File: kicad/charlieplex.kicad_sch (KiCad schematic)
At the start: 244 parts

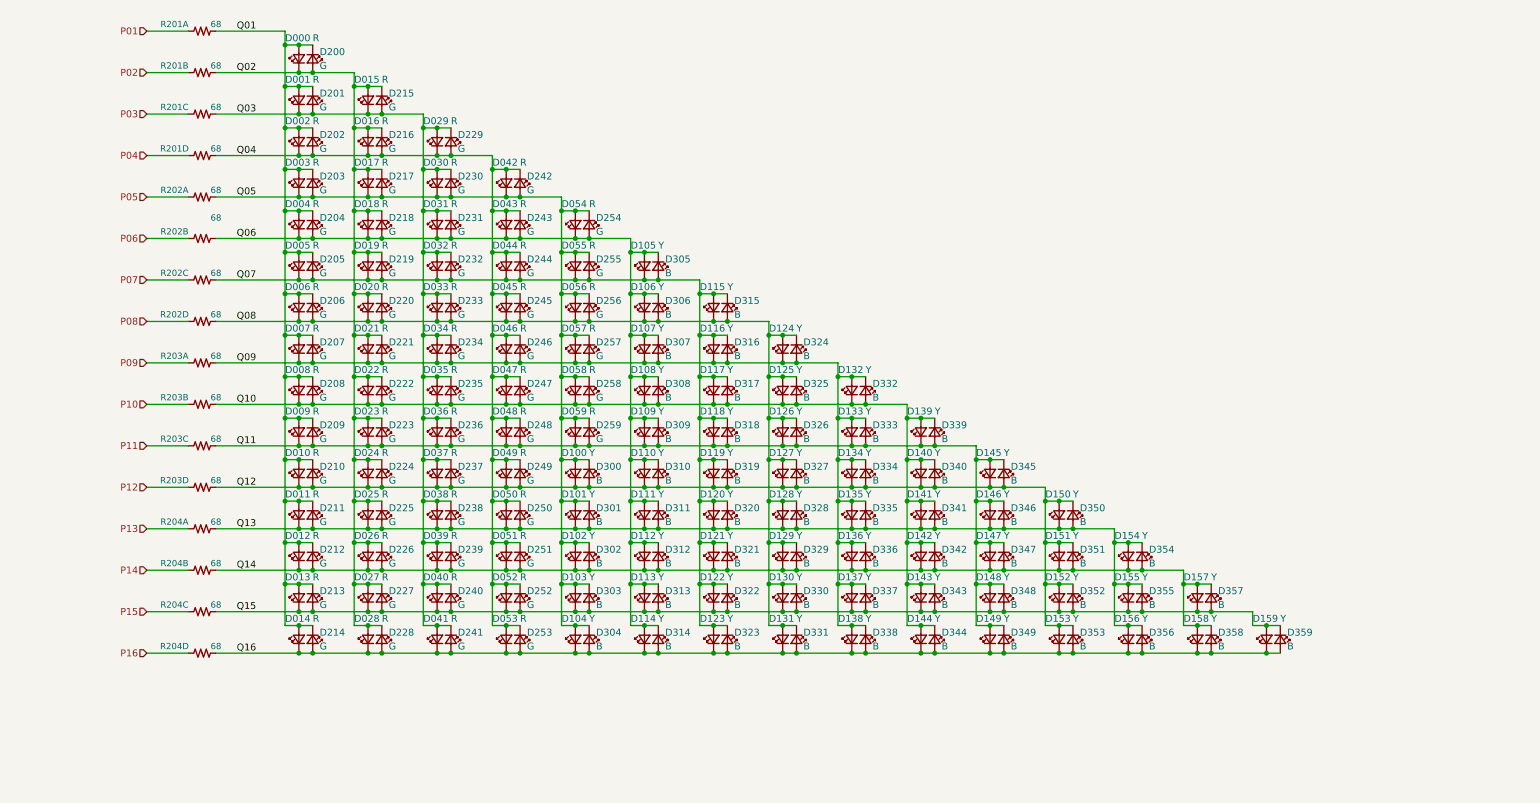
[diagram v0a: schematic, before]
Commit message: Lots of stuff
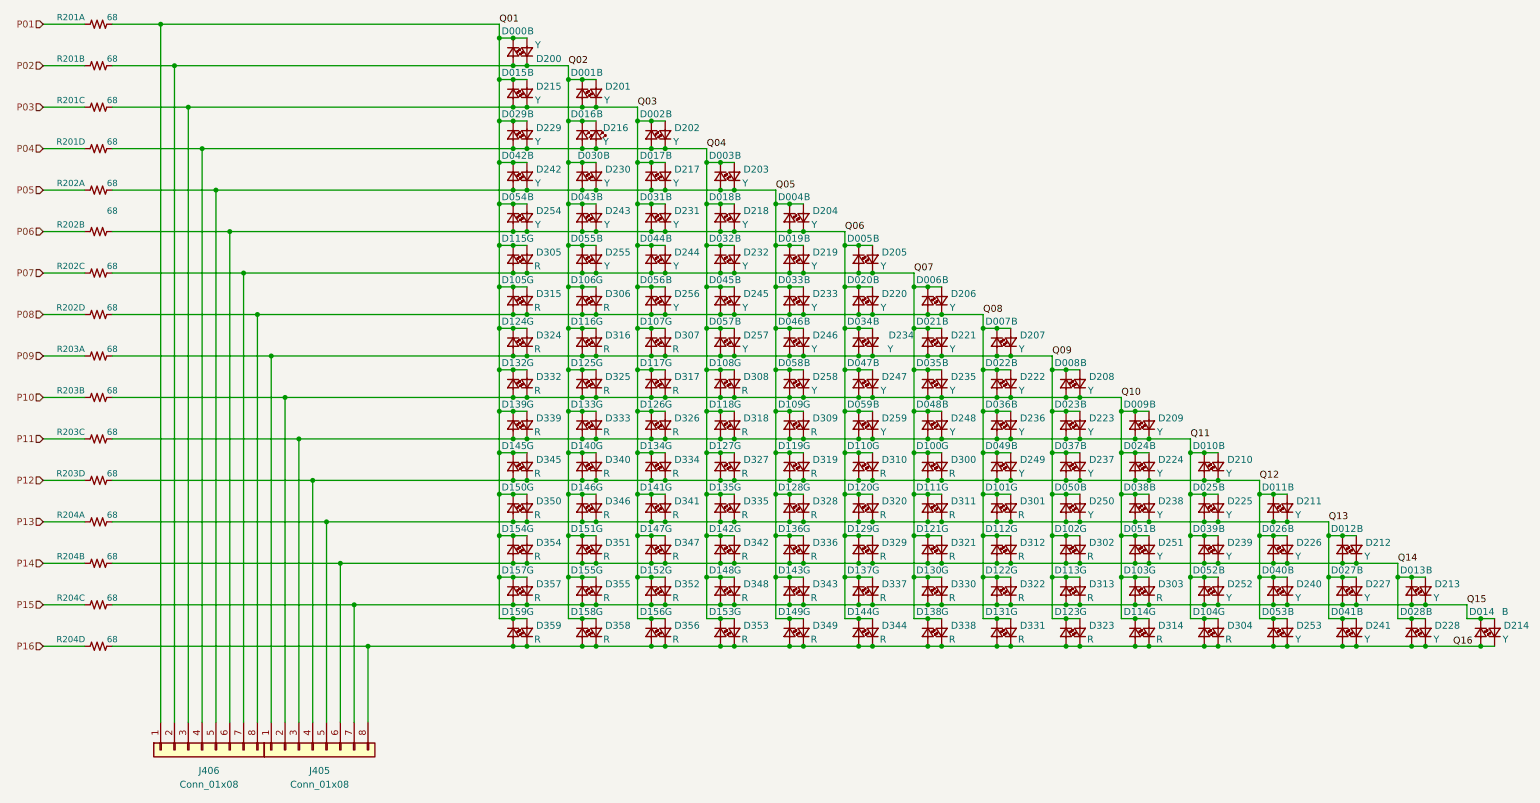
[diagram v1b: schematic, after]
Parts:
- added J405, J406: Conn_01x08, Connector_PinHeader_2.54mm:PinHeader_1x08_P2.54mm_Vertical, symbol Connector_Generic:Conn_01x08
- D000, D001, D002, D003, D004, D005, D006, D007, D008, D009, D010, D011, D012, D013, D014, D015, D016, D017, D018, D019, D020, D021, D022, D023, D024, D025, D026, D027, D028, D029, D030, D031, D032, D033, D034, D035, D036, D037, D038, D039, D040, D041, D042, D043, D044, D045, D046, D047, D048, D049, D050, D051, D052, D053, D054, D055, D056, D057, D058, D059: value R -> B; footprint KwanSystems:D_KINGBRIGHT -> KwanSystems:LED-0603-AC; symbol Device:LED_Small -> KwanSystems:LED_Small_AC; Digikey 754-1816-1-ND -> 754-1789-1-ND; Part Number APGA1602SEC/E/KA -> APT1608VBC/D
- D100, D101, D102, D103, D104, D105, D106, D107, D108, D109, D110, D111, D112, D113, D114, D115, D116, D117, D118, D119, D120, D121, D122, D123, D124, D125, D126, D127, D128, D129, D130, D131, D132, D133, D134, D135, D136, D137, D138, D139, D140, D141, D142, D143, D144, D145, D146, D147, D148, D149, D150, D151, D152, D153, D154, D155, D156, D157, D158, D159: value Y -> G; footprint KwanSystems:D_KINGBRIGHT -> KwanSystems:D_KINGBRIGHT_DOME_AC; symbol Device:LED_Small -> KwanSystems:LED_Small_AC; Digikey 754-1816-1-ND -> 754-2334-1-ND; Part Number APGA1602SEC/E/KA -> APDA1806ZGCK
- D200, D201, D202, D203, D204, D205, D206, D207, D208, D209, D210, D211, D212, D213, D214, D215, D216, D217, D218, D219, D220, D221, D222, D223, D224, D225, D226, D227, D228, D229, D230, D231, D232, D233, D234, D235, D236, D237, D238, D239, D240, D241, D242, D243, D244, D245, D246, D247, D248, D249, D250, D251, D252, D253, D254, D255, D256, D257, D258, D259: value G -> Y; footprint KwanSystems:D_KINGBRIGHT -> KwanSystems:D_KINGBRIGHT_DOME_AC; symbol Device:LED_Small -> KwanSystems:LED_Small_AC; Digikey 754-1820-1-ND -> 754-2331-1-ND; Part Number APGA1602CGC/KA -> APDA1806SYCK
- D300, D301, D302, D303, D304, D305, D306, D307, D308, D309, D310, D311, D312, D313, D314, D315, D316, D317, D318, D319, D320, D321, D322, D323, D324, D325, D326, D327, D328, D329, D330, D331, D332, D333, D334, D335, D336, D337, D338, D339, D340, D341, D342, D343, D344, D345, D346, D347, D348, D349, D350, D351, D352, D353, D354, D355, D356, D357, D358, D359: value B -> R; footprint KwanSystems:D_KINGBRIGHT -> KwanSystems:D_KINGBRIGHT_DOME_AC; symbol Device:LED_Small -> KwanSystems:LED_Small_AC; Digikey 754-1820-1-ND -> 754-2330-1-ND; Part Number APGA1602CGC/KA -> APDA1806SURCK
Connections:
- net Q01: now also D000.C, D015.C, D029.C, D042.C, D054.C, D105.C, D115.C, D124.C, D132.C, D139.C, D145.C, D150.C, D154.C, D157.C, D159.C, D200.A, D215.A, D229.A, D242.A, D254.A, D305.A, D315.A, D324.A, D332.A, D339.A, D345.A, D350.A, D354.A, D357.A, D359.A, J406.1 (Pin_1); no longer D000.2 (A), D001.2 (A), D002.2 (A), D003.2 (A), D004.2 (A), D005.2 (A), D006.2 (A), D007.2 (A), D008.2 (A), D009.2 (A), D010.2 (A), D011.2 (A), D012.2 (A), D013.2 (A), D014.2 (A), D200.1 (K), D201.1 (K), D202.1 (K), D203.1 (K), D204.1 (K), D205.1 (K), D206.1 (K), D207.1 (K), D208.1 (K), D209.1 (K), D210.1 (K), D211.1 (K), D212.1 (K), D213.1 (K), D214.1 (K)
- net Q02: now also D000.A, D001.C, D016.C, D030.C, D043.C, D055.C, D106.C, D116.C, D125.C, D133.C, D140.C, D146.C, D151.C, D155.C, D158.C, D200.C, D201.A, D216.C, D230.A, D243.A, D255.A, D306.A, D316.A, D325.A, D333.A, D340.A, D346.A, D351.A, D355.A, D358.A, J406.2 (Pin_2); no longer D000.1 (K), D015.2 (A), D016.2 (A), D017.2 (A), D018.2 (A), D019.2 (A), D020.2 (A), D021.2 (A), D022.2 (A), D023.2 (A), D024.2 (A), D025.2 (A), D026.2 (A), D027.2 (A), D028.2 (A), D200.2 (A), D215.1 (K), D216.1 (K), D217.1 (K), D218.1 (K), D219.1 (K), D220.1 (K), D221.1 (K), D222.1 (K), D223.1 (K), D224.1 (K), D225.1 (K), D226.1 (K), D227.1 (K), D228.1 (K)
- net Q03: now also D001.A, D002.C, D015.A, D017.C, D031.C, D044.C, D056.C, D107.C, D117.C, D126.C, D134.C, D141.C, D147.C, D152.C, D156.C, D201.C, D202.A, D215.C, D217.A, D231.A, D244.A, D256.A, D307.A, D317.A, D326.A, D334.A, D341.A, D347.A, D352.A, D356.A, J406.3 (Pin_3); no longer D001.1 (K), D015.1 (K), D029.2 (A), D030.2 (A), D031.2 (A), D032.2 (A), D033.2 (A), D034.2 (A), D035.2 (A), D036.2 (A), D037.2 (A), D038.2 (A), D039.2 (A), D040.2 (A), D041.2 (A), D201.2 (A), D215.2 (A), D229.1 (K), D230.1 (K), D231.1 (K), D232.1 (K), D233.1 (K), D234.1 (K), D235.1 (K), D236.1 (K), D237.1 (K), D238.1 (K), D239.1 (K), D240.1 (K), D241.1 (K)
- net Q04: now also D002.A, D003.C, D016.A, D018.C, D029.A, D032.C, D045.C, D057.C, D108.C, D118.C, D127.C, D135.C, D142.C, D148.C, D153.C, D202.C, D203.A, D216.A, D218.A, D229.C, D232.A, D245.A, D257.A, D308.A, D318.A, D327.A, D335.A, D342.A, D348.A, D353.A, J406.4 (Pin_4); no longer D002.1 (K), D016.1 (K), D029.1 (K), D042.2 (A), D043.2 (A), D044.2 (A), D045.2 (A), D046.2 (A), D047.2 (A), D048.2 (A), D049.2 (A), D050.2 (A), D051.2 (A), D052.2 (A), D053.2 (A), D202.2 (A), D216.2 (A), D229.2 (A), D242.1 (K), D243.1 (K), D244.1 (K), D245.1 (K), D246.1 (K), D247.1 (K), D248.1 (K), D249.1 (K), D250.1 (K), D251.1 (K), D252.1 (K), D253.1 (K)
- net Q05: now also D003.A, D004.C, D017.A, D019.C, D030.A, D033.C, D042.A, D046.C, D058.C, D109.C, D119.C, D128.C, D136.C, D143.C, D149.C, D203.C, D204.A, D217.C, D219.A, D230.C, D233.A, D242.C, D246.A, D258.A, D309.A, D319.A, D328.A, D336.A, D343.A, D349.A, J406.5 (Pin_5); no longer D003.1 (K), D017.1 (K), D030.1 (K), D042.1 (K), D054.2 (A), D055.2 (A), D056.2 (A), D057.2 (A), D058.2 (A), D059.2 (A), D100.2 (A), D101.2 (A), D102.2 (A), D103.2 (A), D104.2 (A), D203.2 (A), D217.2 (A), D230.2 (A), D242.2 (A), D254.1 (K), D255.1 (K), D256.1 (K), D257.1 (K), D258.1 (K), D259.1 (K), D300.1 (K), D301.1 (K), D302.1 (K), D303.1 (K), D304.1 (K)
- net Q06: now also D004.A, D005.C, D018.A, D020.C, D031.A, D034.C, D043.A, D047.C, D054.A, D059.C, D110.C, D120.C, D129.C, D137.C, D144.C, D204.C, D205.A, D218.C, D220.A, D231.C, D234.A, D243.C, D247.A, D254.C, D259.A, D310.A, D320.A, D329.A, D337.A, D344.A, J406.6 (Pin_6); no longer D004.1 (K), D018.1 (K), D031.1 (K), D043.1 (K), D054.1 (K), D105.2 (A), D106.2 (A), D107.2 (A), D108.2 (A), D109.2 (A), D110.2 (A), D111.2 (A), D112.2 (A), D113.2 (A), D114.2 (A), D204.2 (A), D218.2 (A), D231.2 (A), D243.2 (A), D254.2 (A), D305.1 (K), D306.1 (K), D307.1 (K), D308.1 (K), D309.1 (K), D310.1 (K), D311.1 (K), D312.1 (K), D313.1 (K), D314.1 (K)
- net Q07: now also D005.A, D006.C, D019.A, D021.C, D032.A, D035.C, D044.A, D048.C, D055.A, D100.C, D105.A, D111.C, D121.C, D130.C, D138.C, D205.C, D206.A, D219.C, D221.A, D232.C, D235.A, D244.C, D248.A, D255.C, D300.A, D305.C, D311.A, D321.A, D330.A, D338.A, J406.7 (Pin_7); no longer D005.1 (K), D019.1 (K), D032.1 (K), D044.1 (K), D055.1 (K), D105.1 (K), D115.2 (A), D116.2 (A), D117.2 (A), D118.2 (A), D119.2 (A), D120.2 (A), D121.2 (A), D122.2 (A), D123.2 (A), D205.2 (A), D219.2 (A), D232.2 (A), D244.2 (A), D255.2 (A), D305.2 (A), D315.1 (K), D316.1 (K), D317.1 (K), D318.1 (K), D319.1 (K), D320.1 (K), D321.1 (K), D322.1 (K), D323.1 (K)
- net Q08: now also D006.A, D007.C, D020.A, D022.C, D033.A, D036.C, D045.A, D049.C, D056.A, D101.C, D106.A, D112.C, D115.A, D122.C, D131.C, D206.C, D207.A, D220.C, D222.A, D233.C, D236.A, D245.C, D249.A, D256.C, D301.A, D306.C, D312.A, D315.C, D322.A, D331.A, J406.8 (Pin_8); no longer D006.1 (K), D020.1 (K), D033.1 (K), D045.1 (K), D056.1 (K), D106.1 (K), D115.1 (K), D124.2 (A), D125.2 (A), D126.2 (A), D127.2 (A), D128.2 (A), D129.2 (A), D130.2 (A), D131.2 (A), D206.2 (A), D220.2 (A), D233.2 (A), D245.2 (A), D256.2 (A), D306.2 (A), D315.2 (A), D324.1 (K), D325.1 (K), D326.1 (K), D327.1 (K), D328.1 (K), D329.1 (K), D330.1 (K), D331.1 (K)
- net Q09: now also D007.A, D008.C, D021.A, D023.C, D034.A, D037.C, D046.A, D050.C, D057.A, D102.C, D107.A, D113.C, D116.A, D123.C, D124.A, D207.C, D208.A, D221.C, D223.A, D234.C, D237.A, D246.C, D250.A, D257.C, D302.A, D307.C, D313.A, D316.C, D323.A, D324.C, J405.1 (Pin_1); no longer D007.1 (K), D021.1 (K), D034.1 (K), D046.1 (K), D057.1 (K), D107.1 (K), D116.1 (K), D124.1 (K), D132.2 (A), D133.2 (A), D134.2 (A), D135.2 (A), D136.2 (A), D137.2 (A), D138.2 (A), D207.2 (A), D221.2 (A), D234.2 (A), D246.2 (A), D257.2 (A), D307.2 (A), D316.2 (A), D324.2 (A), D332.1 (K), D333.1 (K), D334.1 (K), D335.1 (K), D336.1 (K), D337.1 (K), D338.1 (K)
- net Q10: now also D008.A, D009.C, D022.A, D024.C, D035.A, D038.C, D047.A, D051.C, D058.A, D103.C, D108.A, D114.C, D117.A, D125.A, D132.A, D208.C, D209.A, D222.C, D224.A, D235.C, D238.A, D247.C, D251.A, D258.C, D303.A, D308.C, D314.A, D317.C, D325.C, D332.C, J405.2 (Pin_2); no longer D008.1 (K), D022.1 (K), D035.1 (K), D047.1 (K), D058.1 (K), D108.1 (K), D117.1 (K), D125.1 (K), D132.1 (K), D139.2 (A), D140.2 (A), D141.2 (A), D142.2 (A), D143.2 (A), D144.2 (A), D208.2 (A), D222.2 (A), D235.2 (A), D247.2 (A), D258.2 (A), D308.2 (A), D317.2 (A), D325.2 (A), D332.2 (A), D339.1 (K), D340.1 (K), D341.1 (K), D342.1 (K), D343.1 (K), D344.1 (K)
- net Q11: now also D009.A, D010.C, D023.A, D025.C, D036.A, D039.C, D048.A, D052.C, D059.A, D104.C, D109.A, D118.A, D126.A, D133.A, D139.A, D209.C, D210.A, D223.C, D225.A, D236.C, D239.A, D248.C, D252.A, D259.C, D304.A, D309.C, D318.C, D326.C, D333.C, D339.C, J405.3 (Pin_3); no longer D009.1 (K), D023.1 (K), D036.1 (K), D048.1 (K), D059.1 (K), D109.1 (K), D118.1 (K), D126.1 (K), D133.1 (K), D139.1 (K), D145.2 (A), D146.2 (A), D147.2 (A), D148.2 (A), D149.2 (A), D209.2 (A), D223.2 (A), D236.2 (A), D248.2 (A), D259.2 (A), D309.2 (A), D318.2 (A), D326.2 (A), D333.2 (A), D339.2 (A), D345.1 (K), D346.1 (K), D347.1 (K), D348.1 (K), D349.1 (K)
- net Q12: now also D010.A, D011.C, D024.A, D026.C, D037.A, D040.C, D049.A, D053.C, D100.A, D110.A, D119.A, D127.A, D134.A, D140.A, D145.A, D210.C, D211.A, D224.C, D226.A, D237.C, D240.A, D249.C, D253.A, D300.C, D310.C, D319.C, D327.C, D334.C, D340.C, D345.C, J405.4 (Pin_4); no longer D010.1 (K), D024.1 (K), D037.1 (K), D049.1 (K), D100.1 (K), D110.1 (K), D119.1 (K), D127.1 (K), D134.1 (K), D140.1 (K), D145.1 (K), D150.2 (A), D151.2 (A), D152.2 (A), D153.2 (A), D210.2 (A), D224.2 (A), D237.2 (A), D249.2 (A), D300.2 (A), D310.2 (A), D319.2 (A), D327.2 (A), D334.2 (A), D340.2 (A), D345.2 (A), D350.1 (K), D351.1 (K), D352.1 (K), D353.1 (K)
- net Q13: now also D011.A, D012.C, D025.A, D027.C, D038.A, D041.C, D050.A, D101.A, D111.A, D120.A, D128.A, D135.A, D141.A, D146.A, D150.A, D211.C, D212.A, D225.C, D227.A, D238.C, D241.A, D250.C, D301.C, D311.C, D320.C, D328.C, D335.C, D341.C, D346.C, D350.C, J405.5 (Pin_5); no longer D011.1 (K), D025.1 (K), D038.1 (K), D050.1 (K), D101.1 (K), D111.1 (K), D120.1 (K), D128.1 (K), D135.1 (K), D141.1 (K), D146.1 (K), D150.1 (K), D154.2 (A), D155.2 (A), D156.2 (A), D211.2 (A), D225.2 (A), D238.2 (A), D250.2 (A), D301.2 (A), D311.2 (A), D320.2 (A), D328.2 (A), D335.2 (A), D341.2 (A), D346.2 (A), D350.2 (A), D354.1 (K), D355.1 (K), D356.1 (K)
- net Q14: now also D012.A, D013.C, D026.A, D028.C, D039.A, D051.A, D102.A, D112.A, D121.A, D129.A, D136.A, D142.A, D147.A, D151.A, D154.A, D212.C, D213.A, D226.C, D228.A, D239.C, D251.C, D302.C, D312.C, D321.C, D329.C, D336.C, D342.C, D347.C, D351.C, D354.C, J405.6 (Pin_6); no longer D012.1 (K), D026.1 (K), D039.1 (K), D051.1 (K), D102.1 (K), D112.1 (K), D121.1 (K), D129.1 (K), D136.1 (K), D142.1 (K), D147.1 (K), D151.1 (K), D154.1 (K), D157.2 (A), D158.2 (A), D212.2 (A), D226.2 (A), D239.2 (A), D251.2 (A), D302.2 (A), D312.2 (A), D321.2 (A), D329.2 (A), D336.2 (A), D342.2 (A), D347.2 (A), D351.2 (A), D354.2 (A), D357.1 (K), D358.1 (K)
- net Q15: now also D013.A, D014.C, D027.A, D040.A, D052.A, D103.A, D113.A, D122.A, D130.A, D137.A, D143.A, D148.A, D152.A, D155.A, D157.A, D213.C, D214.A, D227.C, D240.C, D252.C, D303.C, D313.C, D322.C, D330.C, D337.C, D343.C, D348.C, D352.C, D355.C, D357.C, J405.7 (Pin_7); no longer D013.1 (K), D027.1 (K), D040.1 (K), D052.1 (K), D103.1 (K), D113.1 (K), D122.1 (K), D130.1 (K), D137.1 (K), D143.1 (K), D148.1 (K), D152.1 (K), D155.1 (K), D157.1 (K), D159.2 (A), D213.2 (A), D227.2 (A), D240.2 (A), D252.2 (A), D303.2 (A), D313.2 (A), D322.2 (A), D330.2 (A), D337.2 (A), D343.2 (A), D348.2 (A), D352.2 (A), D355.2 (A), D357.2 (A), D359.1 (K)
- net Q16: now also D014.A, D028.A, D041.A, D053.A, D104.A, D114.A, D123.A, D131.A, D138.A, D144.A, D149.A, D153.A, D156.A, D158.A, D159.A, D214.C, D228.C, D241.C, D253.C, D304.C, D314.C, D323.C, D331.C, D338.C, D344.C, D349.C, D353.C, D356.C, D358.C, D359.C, J405.8 (Pin_8); no longer D014.1 (K), D028.1 (K), D041.1 (K), D053.1 (K), D104.1 (K), D114.1 (K), D123.1 (K), D131.1 (K), D138.1 (K), D144.1 (K), D149.1 (K), D153.1 (K), D156.1 (K), D158.1 (K), D159.1 (K), D214.2 (A), D228.2 (A), D241.2 (A), D253.2 (A), D304.2 (A), D314.2 (A), D323.2 (A), D331.2 (A), D338.2 (A), D344.2 (A), D349.2 (A), D353.2 (A), D356.2 (A), D358.2 (A), D359.2 (A)
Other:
- moved on the sheet: D000, D001, D002, D003, D004, D005, D006, D007, D008, D009, D010, D011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
